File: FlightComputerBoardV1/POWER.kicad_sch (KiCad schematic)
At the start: 44 parts, among them U14 TPS56A37RPAR, U7 TPS56A37RPAR

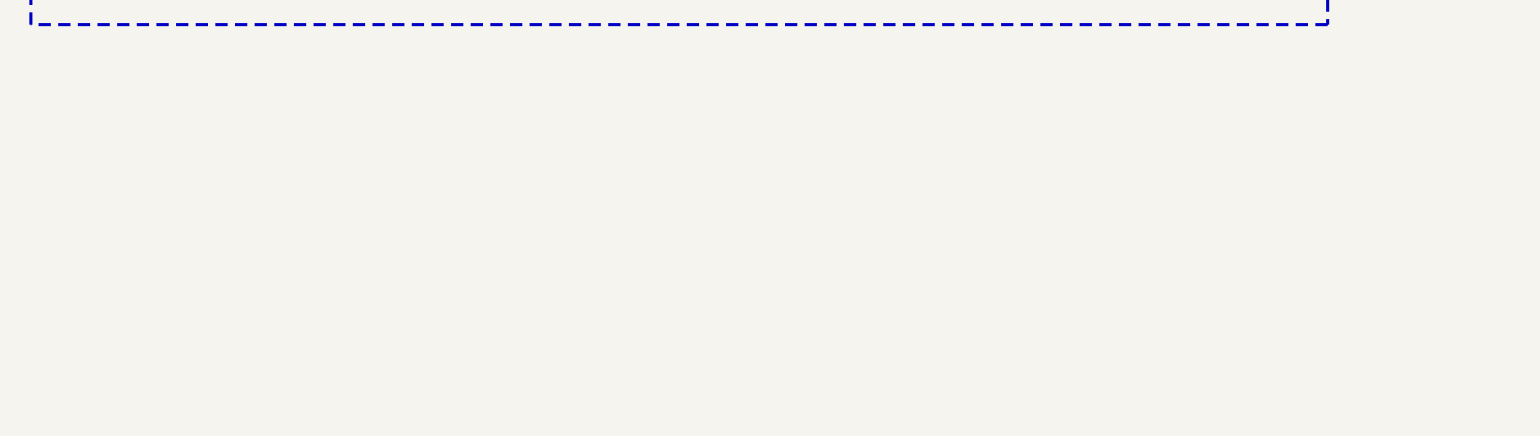
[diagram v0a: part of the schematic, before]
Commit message: temp and power sensor
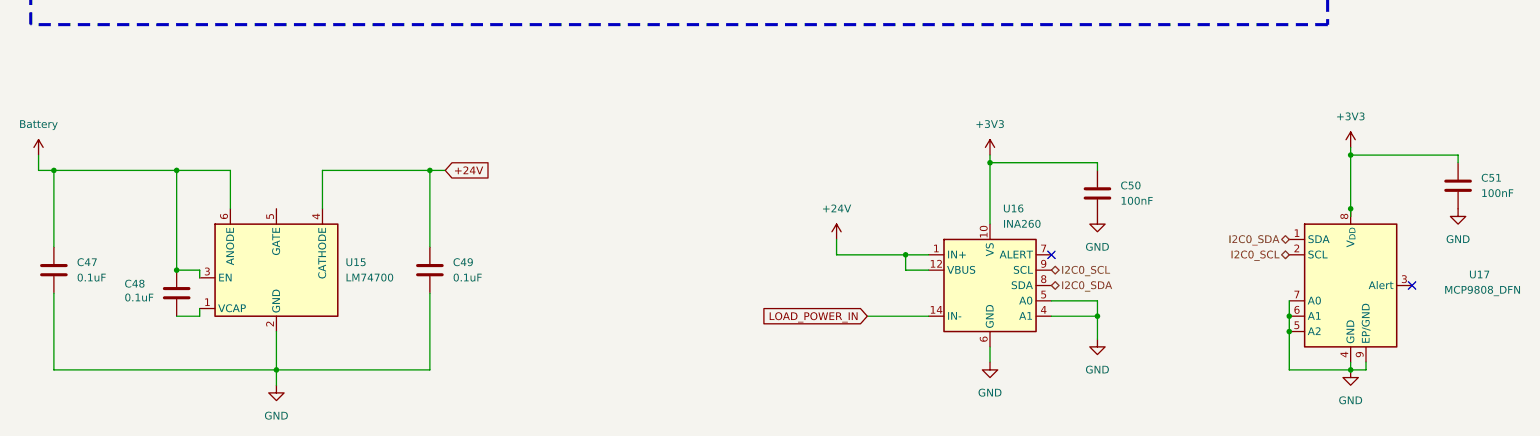
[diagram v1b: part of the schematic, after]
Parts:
- added C47, C48, C49: 0.1uF, symbol Device:C
- added C50, C51: 100nF, symbol Device:C
- added U15: LM74700, Package_TO_SOT_SMD:SOT-23-6, symbol Power_Management:LM74700
- added U16: INA260, Package_SO:TSSOP-16_4.4x5mm_P0.65mm, symbol Sensor_Energy:INA260
- added U17: MCP9808_DFN, Package_DFN_QFN:DFN-8-1EP_3x2mm_P0.5mm_EP1.7x1.4mm, symbol Sensor_Temperature:MCP9808_DFN
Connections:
- net +24V: now also C49.1, U15.4 (CATHODE), U16.1 (IN+), U16.12 (VBUS), U16.2 (IN+), U16.3 (IN+)
- new net: C48.2, U15.1 (VCAP)
- new net +3V3: C50.1, C51.1, U16.10 (VS), U17.8 (V_{DD})
- new net Battery: C47.1, C48.1, U15.3 (EN), U15.6 (ANODE)
- new net GND: C47.2, C49.2, C50.2, C51.2, U15.2 (GND), U16.11 (GND), U16.4 (A1), U16.5 (A0), U16.6 (GND), U17.4 (GND), U17.5 (A2), U17.6 (A1), U17.7 (A0), U17.9 (EP/GND)
- new net I2C0_SCL: U16.9 (SCL), U17.2 (SCL)
- new net I2C0_SDA: U16.8 (SDA), U17.1 (SDA)
- new net LOAD_POWER_IN: U16.14 (IN-), U16.15 (IN-), U16.16 (IN-)
- no-connect marks 0 -> 2
